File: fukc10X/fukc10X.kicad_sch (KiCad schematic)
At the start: 25 parts, among them J1 SM04B-SRSS-TB, J2 Conn_01x02_Pin, J3 Conn_01x02_Pin, J4 Conn_01x02_Pin, J5 Conn_01x02_Pin, J6 Conn_01x02_Pin, J7 Conn_01x02_Pin, J8 Conn_01x02_Pin, U1 XC6206P332MR, U2 STM32F072CBT6

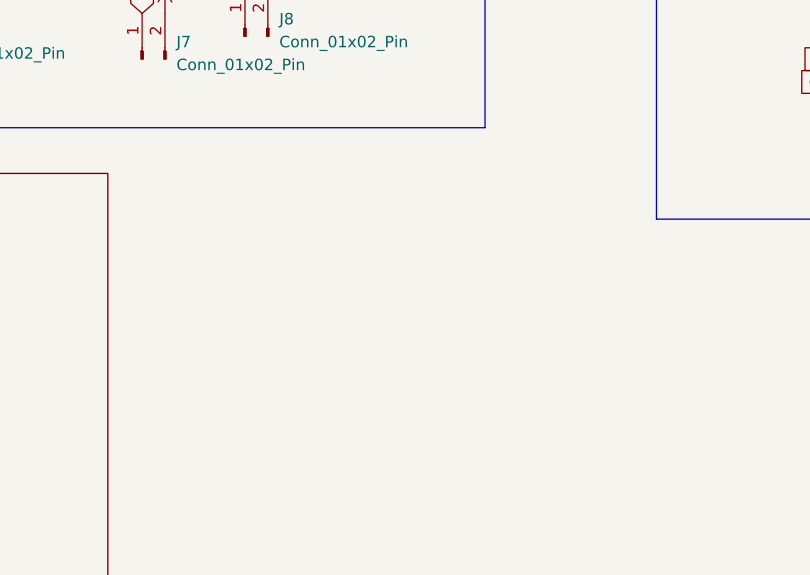
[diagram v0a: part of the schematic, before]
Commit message: Added some Silkscreen Text aswell as spare diodes
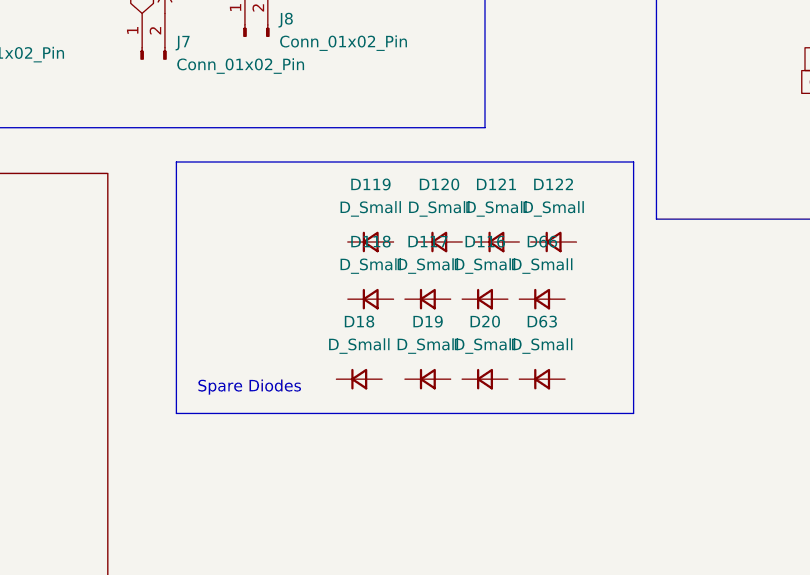
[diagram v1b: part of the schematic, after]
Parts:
- added D116, D117, D118, D119, D120, D121, D122, D18, D19, D20, D63, D66: D_Small, Diode_SMD:D_SOD-123, symbol Device:D_Small
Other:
- note added: "Spare Diodes"
